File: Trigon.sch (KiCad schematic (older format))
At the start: 70 parts, among them J1 USB_C_Receptacle_USB2.0, SW1 SW_Push, SW2 Rotary_Encoder_Switch, U1 ATmega32U4-AU, Y1 16MHz

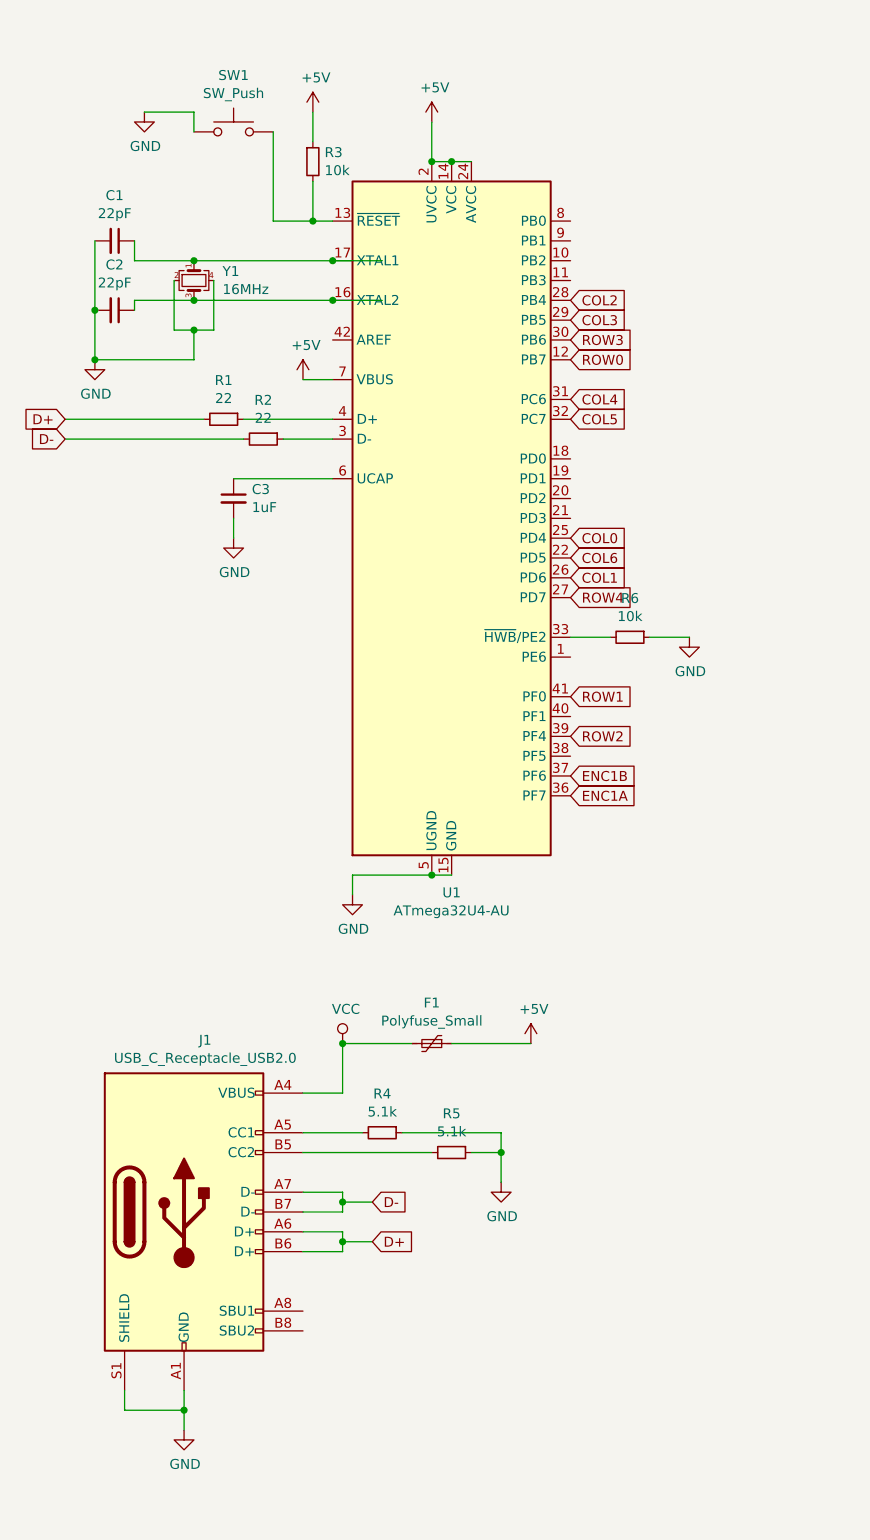
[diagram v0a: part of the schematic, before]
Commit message: new usb connector'
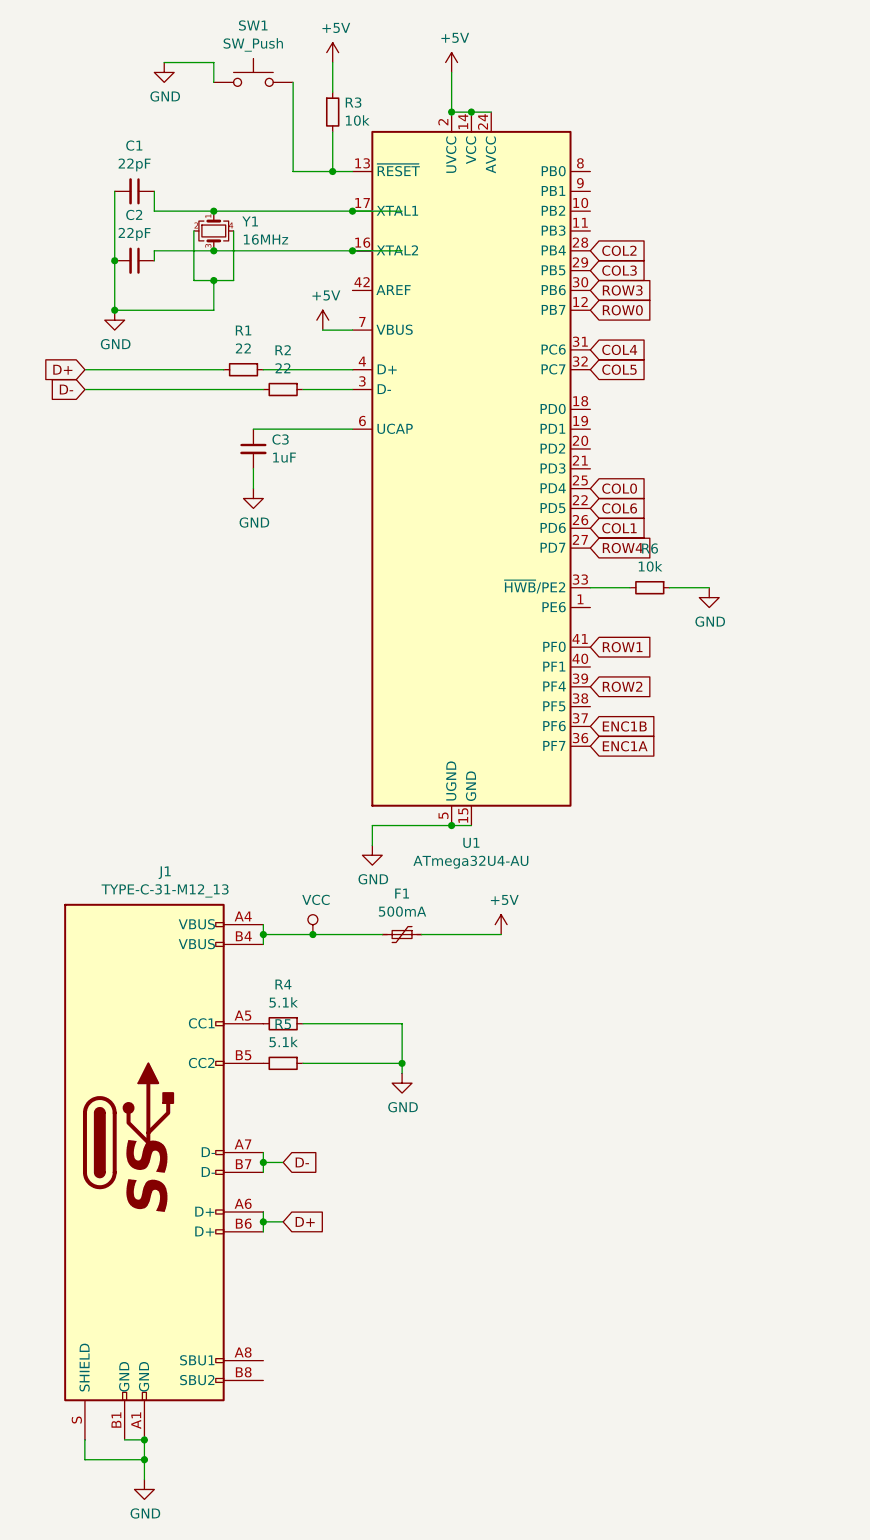
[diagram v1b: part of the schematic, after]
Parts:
- removed J1: USB_C_Receptacle_USB2.0, Connector_USB:USB_C_Receptacle_Palconn_UTC16-G, symbol Connector:USB_C_Receptacle_USB2.0
- added J1: TYPE-C-31-M12_13, acheron_Connectors:TYPE-C-31-M-12, symbol acheronSymbols:TYPE-C-31-M12_13
- F1: value Polyfuse_Small -> 500mA
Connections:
- net D+: now also J1.A6 (D+), J1.B6 (D+)
- net D-: now also J1.A7 (D-), J1.B7 (D-)
- net GND: now also J1.A1 (GND), J1.B1 (GND), J1.S (SHIELD)
- net VCC: now also J1.A4 (VBUS), J1.B4 (VBUS)
- net at R4.2: now also J1.A5 (CC1)
- net at R5.2: now also J1.B5 (CC2)
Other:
- moved on the sheet: C1, C2, C3, F1, R1, R2, R3, R4, R5, R6, SW1, U1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

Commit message: Checkpoint
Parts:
- SW2: footprint Rotary_Encoder:RotaryEncoder_Alps_EC12E-Switch_Vertical_H20mm -> Keebio-Parts:RotaryEncoder_Alps_EC11E-Switch_Vertical_H20mm
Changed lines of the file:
@@
 F 0 "SW2" H 10100 2683 50  0000 C CNN
 F 1 "Rotary_Encoder_Switch" H 10100 2774 50  0000 C CNN
-F 2 "Rotary_Encoder:RotaryEncoder_Alps_EC12E-Switch_Vertical_H20mm" H 9950 3210 50  0001 C CNN
+F 2 "Keebio-Parts:RotaryEncoder_Alps_EC11E-Switch_Vertical_H20mm" H 9950 3210 50  0001 C CNN
 F 3 "~" H 10100 3310 50  0001 C CNN
 	1    10100 3050
